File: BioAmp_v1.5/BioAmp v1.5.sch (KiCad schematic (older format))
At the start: 27 parts, among them J1 Conn_01x02_Male, J2 PJ-3062-CO, J4 Conn_01x03_Male, J5 Conn_01x02_Male, J6 Conn_01x02_Male, J7 Conn_01x02_Male, U1 TL074

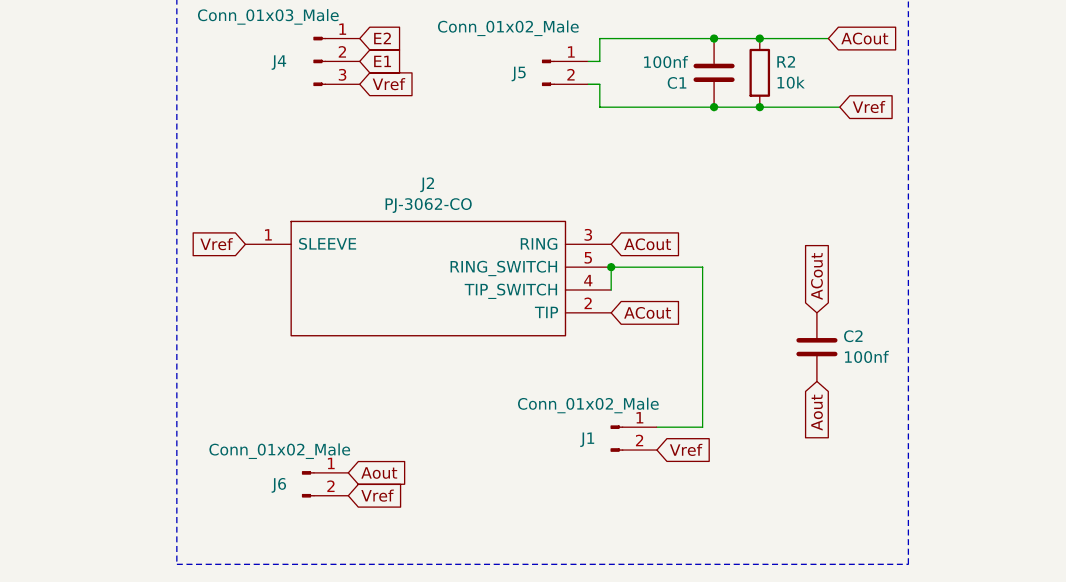
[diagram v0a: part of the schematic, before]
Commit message: update v1.5.4
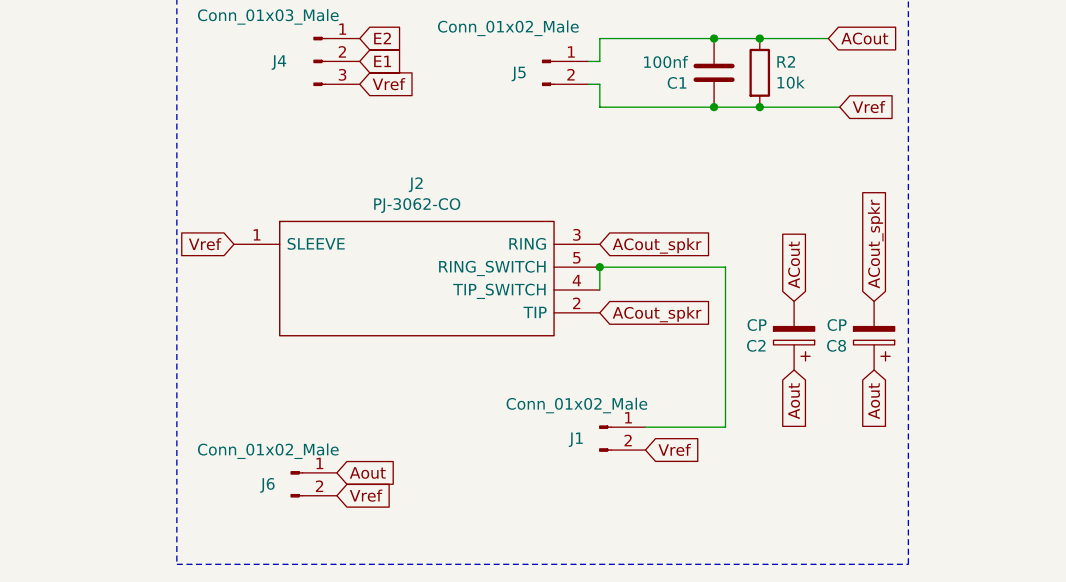
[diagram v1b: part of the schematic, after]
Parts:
- removed C2: 100nf, Capacitor_THT:C_Disc_D3.8mm_W2.6mm_P2.50mm, symbol Device:C
- added C2, C8: CP, Capacitor_THT:CP_Radial_D5.0mm_P2.50mm, symbol Device:CP
- S1: footprint udlabs:TL2285EE -> udlabs:G64_DPDT
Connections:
- net ACout: now also C2.2; no longer J2.2 (TIP), J2.3 (RING)
- net Aout: now also C2.1, C8.1
- new net ACout_spkr: C8.2, J2.2 (TIP), J2.3 (RING)
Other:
- moved on the sheet: J1, J2, J6
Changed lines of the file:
@@
 	1    0    0    -1
 $EndComp
-Text GLabel 3200 6350 2    50   Input ~ 0
+Text GLabel 3150 6350 2    50   Input ~ 0
 Vref
-Text GLabel 3200 6250 2    50   Input ~ 0
+Text GLabel 3150 6250 2    50   Input ~ 0
 Aout
-$Comp
-L Device:C C2
-U 1 1 5FD9D19F
-P 5250 5700
-F 0 "C2" H 5365 5746 50  0000 L CNN
-F 1 "100nf" H 5365 5655 50  0000 L CNN
-F 2 "Capacitor_THT:C_Disc_D3.8mm_W2.6mm_P2.50mm" H 5288 5550 50  0001 C CNN
-F 3 "~" H 5250 5700 50  0001 C CNN
-	1    5250 5700
-	1    0    0    -1
-$EndComp
 $Comp
 L Connector:Conn_01x02_Male J6
 U 1 1 5FD860E1
-P 3000 6250
-F 0 "J6" H 2900 6200 50  0000 C CNN
-F 1 "Conn_01x02_Male" H 2900 6350 50  0000 C CNN
-F 2 "Connector_PinHeader_2.54mm:PinHeader_1x02_P2.54mm_Vertical" H 3000 6250 50  0001 C CNN
-F 3 "~" H 3000 6250 50  0001 C CNN
-	1    3000 6250
-	1    0    0    -1
-$EndComp
-Text GLabel 5250 5850 3    50   Input ~ 0
+P 2950 6250
+F 0 "J6" H 2850 6200 50  0000 C CNN
+F 1 "Conn_01x02_Male" H 2850 6350 50  0000 C CNN
+F 2 "Connector_PinHeader_2.54mm:PinHeader_1x02_P2.54mm_Vertical" H 2950 6250 50  0001 C CNN
+F 3 "~" H 2950 6250 50  0001 C CNN
+	1    2950 6250
+	1    0    0    -1
+$EndComp
+Text GLabel 5150 5800 3    50   Input ~ 0
 Aout
-Text GLabel 5250 5550 1    50   Input ~ 0
+Text GLabel 5150 5500 1    50   Input ~ 0
 ACout
 $Comp
@@
 L Connector:Conn_01x02_Male J1
 U 1 1 5FE44E06
-P 4350 6050
-F 0 "J1" H 4250 6000 50  0000 C CNN
-F 1 "Conn_01x02_Male" H 4250 6150 50  0000 C CNN
-F 2 "Connector_PinHeader_2.54mm:PinHeader_1x02_P2.54mm_Vertical" H 4350 6050 50  0001 C CNN
-F 3 "~" H 4350 6050 50  0001 C CNN
-	1    4350 6050
-	1    0    0    -1
-$EndComp
-Text GLabel 4550 6150 2    50   Input ~ 0
+P 4300 6050
+F 0 "J1" H 4200 6000 50  0000 C CNN
+F 1 "Conn_01x02_Male" H 4200 6150 50  0000 C CNN
+F 2 "Connector_PinHeader_2.54mm:PinHeader_1x02_P2.54mm_Vertical" H 4300 6050 50  0001 C CNN
+F 3 "~" H 4300 6050 50  0001 C CNN
+	1    4300 6050
+	1    0    0    -1
+$EndComp
+Text GLabel 4500 6150 2    50   Input ~ 0
 Vref
 Wire Notes Line
@@
 Wire Notes Line
 	2450 6650 5650 6650
-Wire Notes Line
-	5650 6650 5650 4050
 Wire Notes Line
 	5650 4050 2450 4050
@@
 L udlabs:PJ-3062-CO J2
 U 1 1 6000E706
-P 2750 5500
-F 0 "J2" H 3550 6015 50  0000 C CNN
-F 1 "PJ-3062-CO" H 3550 5924 50  0000 C CNN
-F 2 "udlabs:PJ3062CO" H 4200 5850 50  0001 L CNN
-F 3 "https://datasheet.lcsc.com/szlcsc/1904121407_XKB-Enterprise-PJ-3062-CO_C319113.pdf" H 4200 5750 50  0001 L CNN
-F 4 "Audio & Video Connectors Female DIP RoHS" H 4200 5650 50  0001 L CNN "Description"
-F 5 "11" H 4200 5550 50  0001 L CNN "Height"
-F 6 "XKB Enterprise" H 4200 5450 50  0001 L CNN "Manufacturer_Name"
-F 7 "PJ-3062-CO" H 4200 5350 50  0001 L CNN "Manufacturer_Part_Number"
-	1    2750 5500
-	1    0    0    -1
-$EndComp
-Text GLabel 2750 5250 0    50   Input ~ 0
+P 2700 5500
+F 0 "J2" H 3500 6015 50  0000 C CNN
+F 1 "PJ-3062-CO" H 3500 5924 50  0000 C CNN
+F 2 "udlabs:PJ3062CO" H 4150 5850 50  0001 L CNN
+F 3 "https://datasheet.lcsc.com/szlcsc/1904121407_XKB-Enterprise-PJ-3062-CO_C319113.pdf" H 4150 5750 50  0001 L CNN
+F 4 "Audio & Video Connectors Female DIP RoHS" H 4150 5650 50  0001 L CNN "Description"
+F 5 "11" H 4150 5550 50  0001 L CNN "Height"
+F 6 "XKB Enterprise" H 4150 5450 50  0001 L CNN "Manufacturer_Name"
+F 7 "PJ-3062-CO" H 4150 5350 50  0001 L CNN "Manufacturer_Part_Number"
+	1    2700 5500
+	1    0    0    -1
+$EndComp
+Text GLabel 2700 5250 0    50   Input ~ 0
 Vref
-Text GLabel 4350 5550 2    50   Input ~ 0
-ACout
-Text GLabel 4350 5250 2    50   Input ~ 0
-ACout
+Text GLabel 4300 5550 2    50   Input ~ 0
+ACout_spkr
+Text GLabel 4300 5250 2    50   Input ~ 0
+ACout_spkr
 $Comp
 L Connector:Conn_01x03_Male J4
@@
 Vref
 Wire Wire Line
-	4350 5350 4350 5450
-Wire Wire Line
-	4350 5350 4750 5350
-Wire Wire Line
-	4750 5350 4750 6050
-Wire Wire Line
-	4550 6050 4750 6050
-Connection ~ 4350 5350
+	4300 5350 4300 5450
 $Comp
 L udlabs:TL2285EE S1
@@
 F 0 "S1" H 9050 3515 50  0000 C CNN
 F 1 "TL2285EE" H 9050 3424 50  0000 C CNN
-F 2 "udlabs:TL2285EE" H 9550 3350 50  0001 L CNN
+F 2 "udlabs:G64_DPDT" H 9550 3350 50  0001 L CNN
 F 3 "https://componentsearchengine.com/Datasheets/1/TL2285EE.pdf" H 9550 3250 50  0001 L CNN
 F 4 "Tactile Switches DPDT ALT ACT PC MNT" H 9550 3150 50  0001 L CNN "Description"
@@
 Wire Wire Line
 	7950 3550 7950 3450
+$Comp
+L Device:CP C2
+U 1 1 5FB85B2C
+P 5150 5650
+F 0 "C2" H 5268 5696 50  0000 L CNN
+F 1 "CP" H 5268 5605 50  0000 L CNN
+F 2 "Capacitor_THT:CP_Radial_D5.0mm_P2.50mm" H 5188 5500 50  0001 C CNN
+F 3 "~" H 5150 5650 50  0001 C CNN
+	1    5150 5650
+	-1   0    0    1
+$EndComp
+Wire Wire Line
+	4300 5350 4850 5350
+Wire Wire Line
+	4850 6050 4500 6050
+Connection ~ 4300 5350
+Wire Wire Line
+	4850 5350 4850 6050
+Text GLabel 5500 5500 1    50   Input ~ 0
+ACout_spkr
+Text GLabel 5500 5800 3    50   Input ~ 0
+Aout
+$Comp
+L Device:CP C8
+U 1 1 5FB8EAA6
+P 5500 5650
+F 0 "C8" H 5618 5696 50  0000 L CNN
+F 1 "CP" H 5618 5605 50  0000 L CNN
+F 2 "Capacitor_THT:CP_Radial_D5.0mm_P2.50mm" H 5538 5500 50  0001 C CNN
+F 3 "~" H 5500 5650 50  0001 C CNN
+	1    5500 5650
+	-1   0    0    1
+$EndComp
+Wire Notes Line
+	5650 6650 5650 4050
 $EndSCHEMATC
